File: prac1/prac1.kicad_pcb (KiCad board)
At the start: 2 copper layers, 24.5 x 17 mm, 6 parts, among them J1 Conn_01x01_Pin, J2 Conn_01x01_Pin

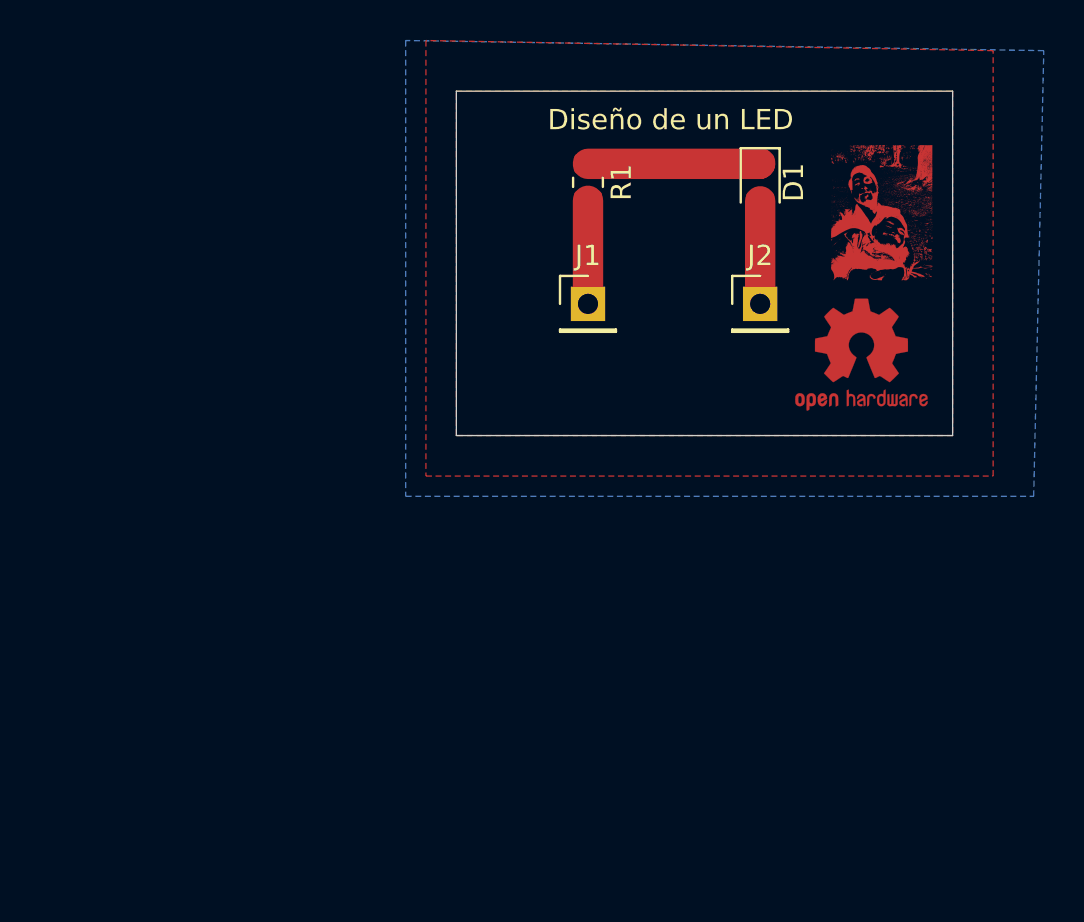
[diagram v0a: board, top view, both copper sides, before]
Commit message: prac 1 2do parcial
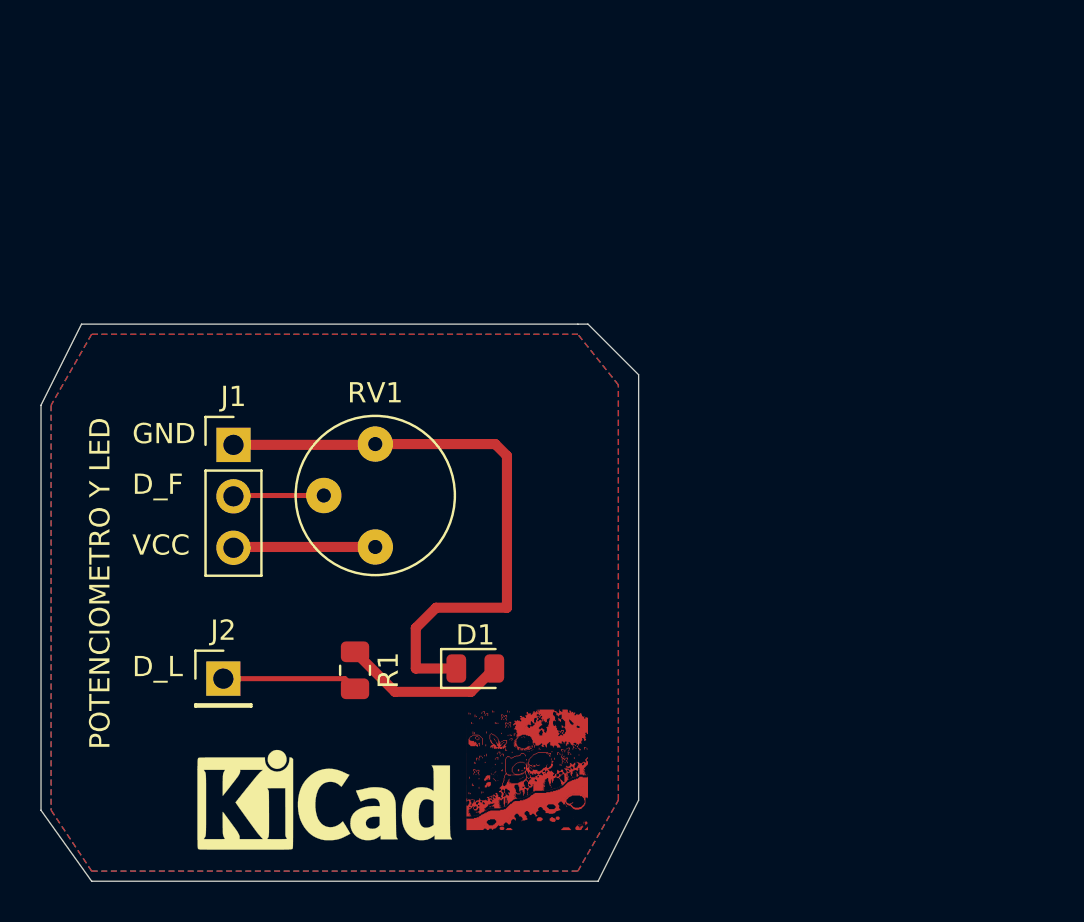
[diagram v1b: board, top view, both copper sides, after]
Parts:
- removed the G*** at (147.5, 81.5)
- removed the REF** at (146.5, 88.5)
- added G***: LOGO, library:fin_logo, F.Cu at (130.0, 109.0)
- added REF**: KiCad-Logo_5mm_SilkScreen, Symbol:KiCad-Logo_5mm_SilkScreen, F.Cu at (120.0, 111.0)
- added RV1: R_Potentiometer, Potentiometer_THT:Potentiometer_Bourns_3339P_Vertical_HandSoldering, F.Cu at (122.5, 98.0)
- J1: value Conn_01x01_Pin -> Conn_01x03_Pin; footprint Connector_PinHeader_2.54mm:PinHeader_1x01_P2.54mm_Vertical -> Connector_PinHeader_2.54mm:PinHeader_1x03_P2.54mm_Vertical
- R1: value 220 -> R
- moved J2 32.3 mm to (115.0, 104.5)
- moved D1 27.8 mm to (127.4, 104.0), turned to 0 degrees
- moved R1 26.7 mm to (121.5, 104.1)
- moved J1 18.8 mm to (115.5, 93.0)
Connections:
- J1 pad 1: Net-(J1-Pin_1) -> GND
- J2 pad 1: Net-(D1-A) -> Net-(J2-Pin_1)
- R1 pad 1: GND -> Net-(D1-A)
- R1 pad 2: Net-(J1-Pin_1) -> Net-(J2-Pin_1)
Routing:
- net GND: track 8.51 -> 30.2 mm
- net Net-(J1-Pin_3): track 0.00 -> 7.02 mm
- net Net-(J2-Pin_1): track 0.00 -> 6.71 mm
- net Net-(J1-Pin_1): track 5.09 -> 0.00 mm
- net Net-(J1-Pin_2): track 0.00 -> 4.48 mm
- net Net-(D1-A): track 5.06 -> 8.17 mm
- added copper zone on B.Cu, net GND
- removed copper zone on B.Cu, net (none)
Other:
- board size 24.5 x 17 mm -> 29.5 x 27.5 mm
- board text added: "D_F"
- board text added: "D_L"
- board text added: "GND"
- board text added: "POTENCIOMETRO Y LED"
- board text added: "VCC"
- board text removed: "Diseño de un LED"
